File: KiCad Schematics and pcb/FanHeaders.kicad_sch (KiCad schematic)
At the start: 10 parts, among them IC3 EMC2101-ACZL-TR, J4 Conn_01x02_Pin, M2 Fan_4pin, M3 Fan_4pin, M4 Fan_4pin, M5 Fan_4pin, Q1 DMN4035L-7, Q2 DMN4035L-7

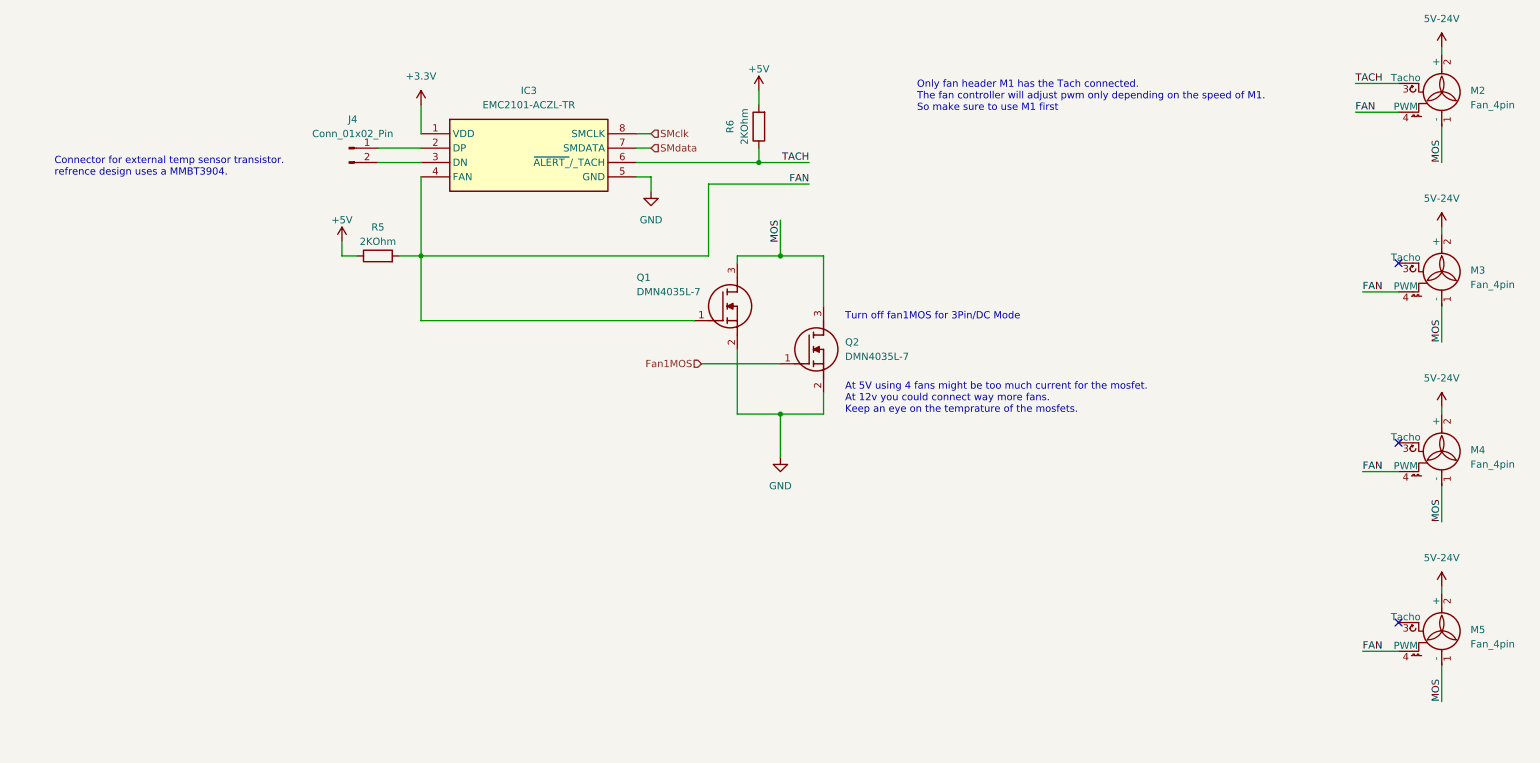
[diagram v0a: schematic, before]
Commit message: v0.1
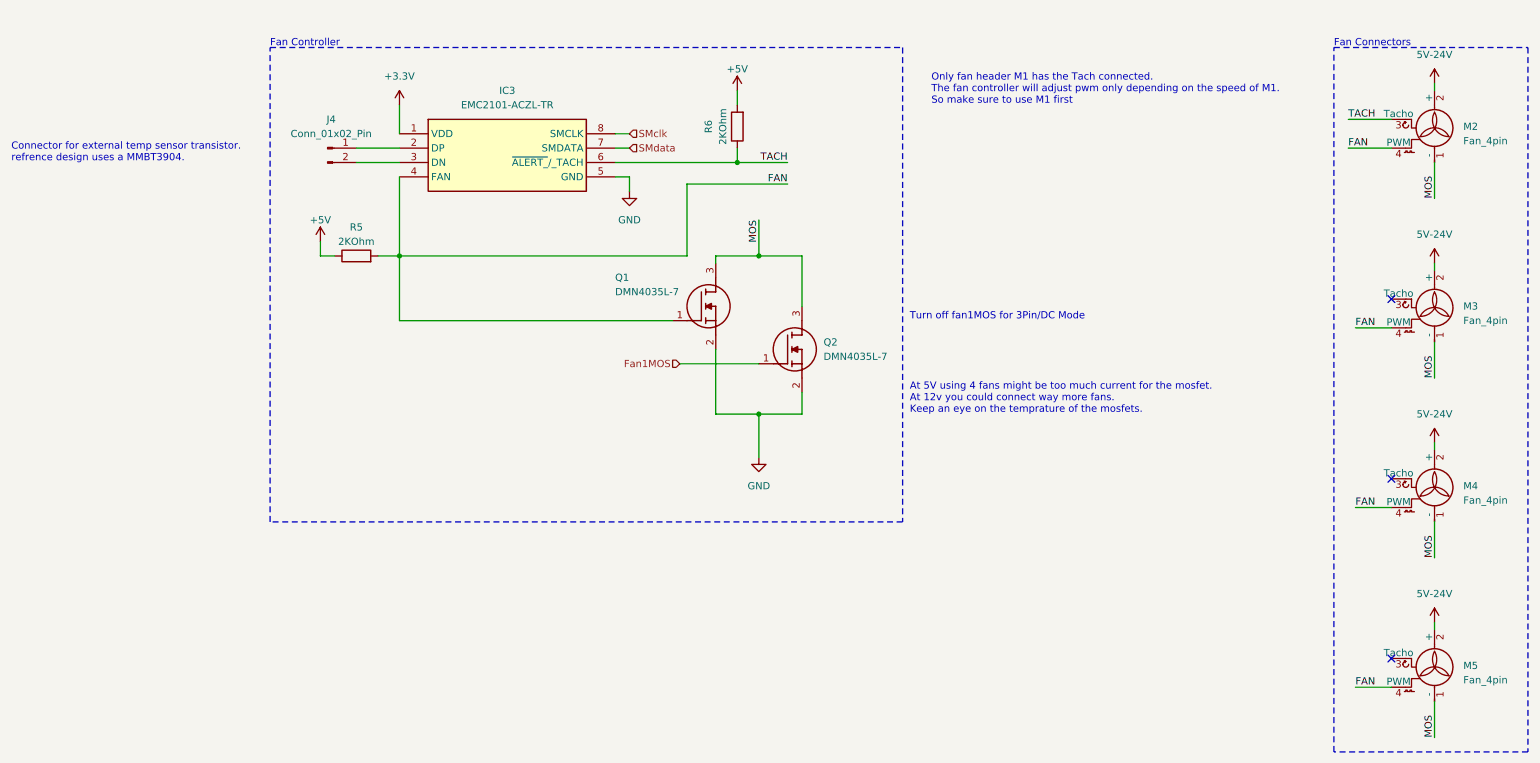
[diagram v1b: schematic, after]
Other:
- note added: "Fan Connectors"
- note added: "Fan Controller"
- moved on the sheet: IC3, J4, M2, M3, M4, M5, Q1, Q2, R5, R6
